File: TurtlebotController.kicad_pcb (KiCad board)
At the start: 2 copper layers, 110 x 80 mm, 80 parts, among them J1 Raspberry_Pi_2_3, J2 LEFT_MOTOR, J3 RIGHT_MOTOR, J4 5V_OUT, J5 3.3V _OUT, J6 12V_OUT, U1 Teensy4.0, U2 MinIMU-9_V5, U3 VNH5019, U4 VNH5019, U5 ACS711xLCTR-25AB, U6 D24V90F5, U7 UltimateSensorFusion_MPU9250_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

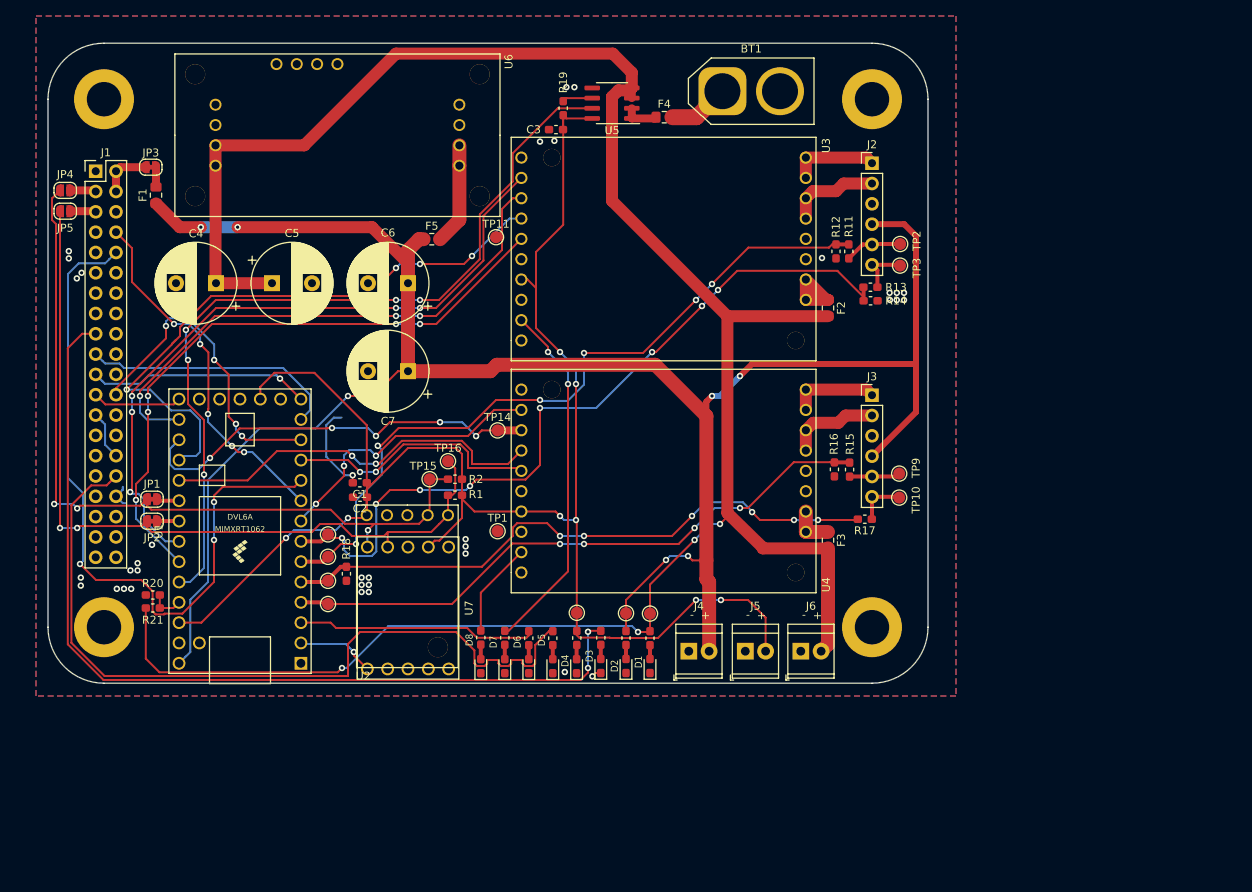
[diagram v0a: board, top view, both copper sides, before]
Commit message: Most of rev B
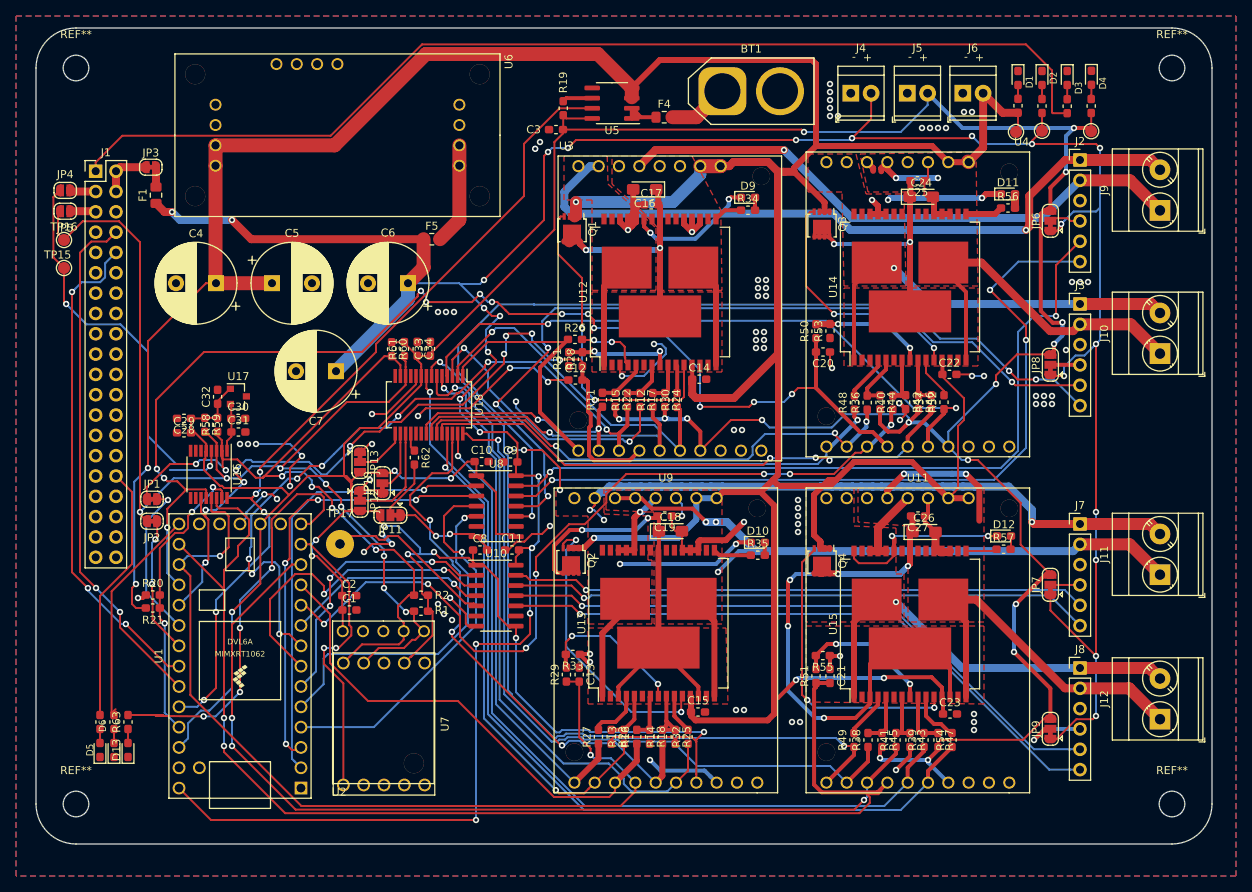
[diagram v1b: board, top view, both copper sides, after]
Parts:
- removed D7: LEFT_MOTOR_OK, LED_SMD:LED_0603_1608Metric_Pad1.05x0.95mm_HandSolder
- removed D8: RIGHT_MOTOR_OK, LED_SMD:LED_0603_1608Metric_Pad1.05x0.95mm_HandSolder
- removed F2, F3: Fuse, Fuse:Fuse_0805_2012Metric_Pad1.15x1.40mm_HandSolder
- removed R10, R9: 500Ohm, Resistor_SMD:R_0603_1608Metric_Pad1.05x0.95mm_HandSolder
- removed the REF** at (78.5, 111.4)
- removed the REF** at (174.5, 111.4)
- removed the REF** at (78.5, 45.4)
- removed the REF** at (174.5, 45.4)
- removed TP1: GND, TestPoint:TestPoint_Pad_D1.5mm
- removed TP10: RIGHT_ENCODER_B_5V, TestPoint:TestPoint_Pad_D1.5mm
- removed TP11: LEFT_PWM, TestPoint:TestPoint_Pad_D1.5mm
- removed TP12: RIGHT_ENCODER_A_3.3V, TestPoint:TestPoint_Pad_D1.5mm
- removed TP13: RIGHT_ENCODER_B_3.3V, TestPoint:TestPoint_Pad_D1.5mm
- removed TP14: RIGHT_PWM, TestPoint:TestPoint_Pad_D1.5mm
- removed TP2: LEFT_ENCODER_A_5V, TestPoint:TestPoint_Pad_D1.5mm
- removed TP3: LEFT_ENCODER_B_5V, TestPoint:TestPoint_Pad_D1.5mm
- removed TP7: LEFT_ENCODER_A_3.3V, TestPoint:TestPoint_Pad_D1.5mm
- removed TP8: LEFT_ENCODER_B_3.3V, TestPoint:TestPoint_Pad_D1.5mm
- removed TP9: RIGHT_ENCODER_A_5V, TestPoint:TestPoint_Pad_D1.5mm
- added C10: 0.1uF, Capacitor_SMD:C_0603_1608Metric_Pad1.05x0.95mm_HandSolder, F.Cu at (125.7, 90.7)
- added C11: 0.1uF, Capacitor_SMD:C_0603_1608Metric_Pad1.05x0.95mm_HandSolder, F.Cu at (129.5, 101.8)
- added C12: 33nF, Capacitor_SMD:C_0603_1608Metric_Pad1.05x0.95mm_HandSolder, F.Cu at (137.4, 80.5)
- added C13: 33nF, Capacitor_SMD:C_0603_1608Metric_Pad1.05x0.95mm_HandSolder, F.Cu at (137.9, 117.3)
- added C14: 0.1uF, Capacitor_SMD:C_0603_1608Metric_Pad1.05x0.95mm_HandSolder, F.Cu at (152.9, 80.4)
- added C15: 0.1uF, Capacitor_SMD:C_0603_1608Metric_Pad1.05x0.95mm_HandSolder, F.Cu at (152.8, 122.0)
- added C16: 47uF, Capacitor_Tantalum_SMD:CP_EIA-3216-10_Kemet-I_Pad1.58x1.35mm_HandSolder, F.Cu at (146.1, 56.7)
- added C17: 0.1uF, Capacitor_SMD:C_0603_1608Metric_Pad1.05x0.95mm_HandSolder, F.Cu at (146.9, 58.6)
- added C18: 47uF, Capacitor_Tantalum_SMD:CP_EIA-3216-10_Kemet-I_Pad1.58x1.35mm_HandSolder, F.Cu at (149.3, 99.4)
- added C19: 0.1uF, Capacitor_SMD:C_0603_1608Metric_Pad1.05x0.95mm_HandSolder, F.Cu at (148.6, 97.5)
- added C20: 33nF, Capacitor_SMD:C_0603_1608Metric_Pad1.05x0.95mm_HandSolder, F.Cu at (168.4, 77.0)
- added C21: 33nF, Capacitor_SMD:C_0603_1608Metric_Pad1.05x0.95mm_HandSolder, F.Cu at (169.2, 117.5)
- added C22: 0.1uF, Capacitor_SMD:C_0603_1608Metric_Pad1.05x0.95mm_HandSolder, F.Cu at (184.2, 79.8)
- added C23: 0.1uF, Capacitor_SMD:C_0603_1608Metric_Pad1.05x0.95mm_HandSolder, F.Cu at (184.2, 122.2)
- added C24: 47uF, Capacitor_Tantalum_SMD:CP_EIA-3216-10_Kemet-I_Pad1.58x1.35mm_HandSolder, F.Cu at (180.7, 57.6)
- added C25: 0.1uF, Capacitor_SMD:C_0603_1608Metric_Pad1.05x0.95mm_HandSolder, F.Cu at (180.2, 55.6)
- added C26: 47uF, Capacitor_Tantalum_SMD:CP_EIA-3216-10_Kemet-I_Pad1.58x1.35mm_HandSolder, F.Cu at (181.0, 99.5)
- added C27: 0.1uF, Capacitor_SMD:C_0603_1608Metric_Pad1.05x0.95mm_HandSolder, F.Cu at (180.2, 97.5)
- added C28: 1uF, Capacitor_SMD:C_0603_1608Metric_Pad1.05x0.95mm_HandSolder, F.Cu at (88.5, 85.3)
- added C29: 0.1uF, Capacitor_SMD:C_0603_1608Metric_Pad1.05x0.95mm_HandSolder, F.Cu at (88.5, 87.1)
- added C30: 0.1uF, Capacitor_SMD:C_0603_1608Metric_Pad1.05x0.95mm_HandSolder, F.Cu at (95.3, 85.3)
- added C31: 1uF, Capacitor_SMD:C_0603_1608Metric_Pad1.05x0.95mm_HandSolder, F.Cu at (95.3, 87.0)
- added C32: 0.47uF, Capacitor_SMD:C_0603_1608Metric_Pad1.05x0.95mm_HandSolder, F.Cu at (92.7, 82.6)
- added C33: 1uF, Capacitor_SMD:C_0603_1608Metric_Pad1.05x0.95mm_HandSolder, F.Cu at (119.3, 76.6)
- added C34: 0.1uF, Capacitor_SMD:C_0603_1608Metric_Pad1.05x0.95mm_HandSolder, F.Cu at (117.7, 76.6)
- added C8: 0.1uF, Capacitor_SMD:C_0603_1608Metric_Pad1.05x0.95mm_HandSolder, F.Cu at (125.5, 101.8)
- added C9: 0.1uF, Capacitor_SMD:C_0603_1608Metric_Pad1.05x0.95mm_HandSolder, F.Cu at (129.3, 90.8)
- added D10: LED_Dual_2pin, LED_SMD:LED_0603_1608Metric_Pad1.05x0.95mm_HandSolder, F.Cu at (160.2, 100.8)
- added D11: LED_Dual_2pin, LED_SMD:LED_0603_1608Metric_Pad1.05x0.95mm_HandSolder, F.Cu at (191.5, 57.2)
- added D12: LED_Dual_2pin, LED_SMD:LED_0603_1608Metric_Pad1.05x0.95mm_HandSolder, F.Cu at (191.0, 100.0)
- added D13: TEENSY_DEBUG, LED_SMD:LED_0603_1608Metric_Pad1.05x0.95mm_HandSolder, F.Cu at (81.5, 126.8)
- added D9: LED_Dual_2pin, LED_SMD:LED_0603_1608Metric_Pad1.05x0.95mm_HandSolder, F.Cu at (159.0, 57.7)
- added J10: Screw_Terminal_01x02, TerminalBlock_Phoenix:TerminalBlock_Phoenix_MKDS-3-2-5.08_1x02_P5.08mm_Horizontal, F.Cu at (210.5, 77.2)
- added J11: Screw_Terminal_01x02, TerminalBlock_Phoenix:TerminalBlock_Phoenix_MKDS-3-2-5.08_1x02_P5.08mm_Horizontal, F.Cu at (210.5, 104.8)
- added J12: Screw_Terminal_01x02, TerminalBlock_Phoenix:TerminalBlock_Phoenix_MKDS-3-2-5.08_1x02_P5.08mm_Horizontal, F.Cu at (210.5, 122.9)
- added J7: MOTOR_3, Connector_PinHeader_2.54mm:PinHeader_1x06_P2.54mm_Vertical, F.Cu at (200.5, 98.5)
- added J8: MOTOR_4, Connector_PinHeader_2.54mm:PinHeader_1x06_P2.54mm_Vertical, F.Cu at (200.5, 116.5)
- added J9: Screw_Terminal_01x02, TerminalBlock_Phoenix:TerminalBlock_Phoenix_MKDS-3-2-5.08_1x02_P5.08mm_Horizontal, F.Cu at (210.5, 59.3)
- added JP10: Jumper_3_Bridged12, Jumper:SolderJumper-3_P1.3mm_Bridged12_RoundedPad1.0x1.5mm, F.Cu at (113.3, 93.4)
- added JP11: Jumper_3_Bridged12, Jumper:SolderJumper-3_P1.3mm_Bridged12_RoundedPad1.0x1.5mm, F.Cu at (114.3, 97.4)
- added JP12: Jumper_3_Bridged12, Jumper:SolderJumper-3_P1.3mm_Bridged12_RoundedPad1.0x1.5mm, F.Cu at (110.5, 95.6)
- added JP13: Jumper_3_Bridged12, Jumper:SolderJumper-3_P1.3mm_Bridged12_RoundedPad1.0x1.5mm, F.Cu at (110.5, 90.8)
- added JP6: Jumper_3_Bridged12, Jumper:SolderJumper-3_P1.3mm_Bridged12_RoundedPad1.0x1.5mm, F.Cu at (196.8, 60.6)
- added JP7: Jumper_3_Bridged12, Jumper:SolderJumper-3_P1.3mm_Bridged12_RoundedPad1.0x1.5mm, F.Cu at (196.8, 106.1)
- added JP8: Jumper_3_Bridged12, Jumper:SolderJumper-3_P1.3mm_Bridged12_RoundedPad1.0x1.5mm, F.Cu at (196.8, 78.6)
- added JP9: Jumper_3_Bridged12, Jumper:SolderJumper-3_P1.3mm_Bridged12_RoundedPad1.0x1.5mm, F.Cu at (196.8, 124.1)
- added Q1: BUK7M12-40EX, Package_TO_SOT_SMD:LFPAK33, F.Cu at (137.0, 61.6)
- added Q2: BUK7M12-40EX, Package_TO_SOT_SMD:LFPAK33, F.Cu at (136.9, 103.0)
- added Q3: BUK7M12-40EX, Package_TO_SOT_SMD:LFPAK33, F.Cu at (168.2, 61.0)
- added Q4: BUK7M12-40EX, Package_TO_SOT_SMD:LFPAK33, F.Cu at (168.2, 103.1)
- added R22: 4.7k, Resistor_SMD:R_0603_1608Metric_Pad1.05x0.95mm_HandSolder, F.Cu at (142.4, 83.0)
- added R23: 4.7k, Resistor_SMD:R_0603_1608Metric_Pad1.05x0.95mm_HandSolder, F.Cu at (141.9, 125.1)
- added R24: 4.7k, Resistor_SMD:R_0603_1608Metric_Pad1.05x0.95mm_HandSolder, F.Cu at (148.6, 83.0)
- added R25: 4.7k, Resistor_SMD:R_0603_1608Metric_Pad1.05x0.95mm_HandSolder, F.Cu at (149.9, 125.1)
- added R26: 1k, Resistor_SMD:R_0603_1608Metric_Pad1.05x0.95mm_HandSolder, F.Cu at (137.4, 75.4)
- added R27: 1k, Resistor_SMD:R_0603_1608Metric_Pad1.05x0.95mm_HandSolder, F.Cu at (140.3, 125.1)
- added R28: 10k, Resistor_SMD:R_0603_1608Metric_Pad1.05x0.95mm_HandSolder, F.Cu at (138.3, 77.9)
- added R29: 10k, Resistor_SMD:R_0603_1608Metric_Pad1.05x0.95mm_HandSolder, F.Cu at (136.3, 117.3)
- added R30: 1k, Resistor_SMD:R_0603_1608Metric_Pad1.05x0.95mm_HandSolder, F.Cu at (150.2, 83.0)
- added R31: 1k, Resistor_SMD:R_0603_1608Metric_Pad1.05x0.95mm_HandSolder, F.Cu at (136.6, 77.9)
- added R32: 1k, Resistor_SMD:R_0603_1608Metric_Pad1.05x0.95mm_HandSolder, F.Cu at (151.5, 125.1)
- added R33: 1k, Resistor_SMD:R_0603_1608Metric_Pad1.05x0.95mm_HandSolder, F.Cu at (137.1, 114.8)
- added R34: 4.7k, Resistor_SMD:R_0603_1608Metric_Pad1.05x0.95mm_HandSolder, F.Cu at (159.0, 59.3)
- added R35: 4.7k, Resistor_SMD:R_0603_1608Metric_Pad1.05x0.95mm_HandSolder, F.Cu at (160.2, 102.4)
- added R36: 1k, Resistor_SMD:R_0603_1608Metric_Pad1.05x0.95mm_HandSolder, F.Cu at (173.9, 83.3)
- added R37: 1k, Resistor_SMD:R_0603_1608Metric_Pad1.05x0.95mm_HandSolder, F.Cu at (181.9, 83.3)
- added R38: 1k, Resistor_SMD:R_0603_1608Metric_Pad1.05x0.95mm_HandSolder, F.Cu at (174.0, 125.5)
- added R39: 1k, Resistor_SMD:R_0603_1608Metric_Pad1.05x0.95mm_HandSolder, F.Cu at (181.0, 125.5)
- added R40: 1k, Resistor_SMD:R_0603_1608Metric_Pad1.05x0.95mm_HandSolder, F.Cu at (177.1, 83.3)
- added R41: 1k, Resistor_SMD:R_0603_1608Metric_Pad1.05x0.95mm_HandSolder, F.Cu at (177.5, 125.5)
- added R42: 10k, Resistor_SMD:R_0603_1608Metric_Pad1.05x0.95mm_HandSolder, F.Cu at (178.7, 83.3)
- added R43: 10k, Resistor_SMD:R_0603_1608Metric_Pad1.05x0.95mm_HandSolder, F.Cu at (179.2, 125.5)
- added R44: 4.7k, Resistor_SMD:R_0603_1608Metric_Pad1.05x0.95mm_HandSolder, F.Cu at (175.5, 83.3)
- added R45: 4.7k, Resistor_SMD:R_0603_1608Metric_Pad1.05x0.95mm_HandSolder, F.Cu at (175.8, 125.5)
- added R46: 4.7k, Resistor_SMD:R_0603_1608Metric_Pad1.05x0.95mm_HandSolder, F.Cu at (180.3, 83.3)
- added R47: 4.7k, Resistor_SMD:R_0603_1608Metric_Pad1.05x0.95mm_HandSolder, F.Cu at (182.8, 125.5)
- added R48: 1k, Resistor_SMD:R_0603_1608Metric_Pad1.05x0.95mm_HandSolder, F.Cu at (172.3, 83.3)
- added R49: 1k, Resistor_SMD:R_0603_1608Metric_Pad1.05x0.95mm_HandSolder, F.Cu at (172.2, 125.5)
- added R50: 10k, Resistor_SMD:R_0603_1608Metric_Pad1.05x0.95mm_HandSolder, F.Cu at (167.5, 74.4)
- added R51: 10k, Resistor_SMD:R_0603_1608Metric_Pad1.05x0.95mm_HandSolder, F.Cu at (167.5, 117.5)
- added R52: 1k, Resistor_SMD:R_0603_1608Metric_Pad1.05x0.95mm_HandSolder, F.Cu at (183.5, 83.3)
- added R53: 1k, Resistor_SMD:R_0603_1608Metric_Pad1.05x0.95mm_HandSolder, F.Cu at (169.2, 74.4)
- added R54: 1k, Resistor_SMD:R_0603_1608Metric_Pad1.05x0.95mm_HandSolder, F.Cu at (184.5, 125.5)
- added R55: 1k, Resistor_SMD:R_0603_1608Metric_Pad1.05x0.95mm_HandSolder, F.Cu at (168.3, 115.0)
- added R56: 4.7k, Resistor_SMD:R_0603_1608Metric_Pad1.05x0.95mm_HandSolder, F.Cu at (191.5, 59.0)
- added R57: 4.7k, Resistor_SMD:R_0603_1608Metric_Pad1.05x0.95mm_HandSolder, F.Cu at (190.9, 101.7)
- added R58: 4.7k, Resistor_SMD:R_0603_1608Metric_Pad1.05x0.95mm_HandSolder, F.Cu at (92.7, 86.1)
- added R59: 4.7k, Resistor_SMD:R_0603_1608Metric_Pad1.05x0.95mm_HandSolder, F.Cu at (91.1, 86.1)
- added R60: 4.7k, Resistor_SMD:R_0603_1608Metric_Pad1.05x0.95mm_HandSolder, F.Cu at (114.5, 76.7)
- added R61: 4.7k, Resistor_SMD:R_0603_1608Metric_Pad1.05x0.95mm_HandSolder, F.Cu at (116.0, 76.6)
- added R62: 4.7k, Resistor_SMD:R_0603_1608Metric_Pad1.05x0.95mm_HandSolder, F.Cu at (117.3, 90.2)
- added R63: 65Ohm, Resistor_SMD:R_0603_1608Metric_Pad1.05x0.95mm_HandSolder, F.Cu at (81.5, 123.2)
- added REF**: MountingHole_3.2mm_M3, MountingHole:MountingHole_3.2mm_M3, F.Cu at (212.0, 133.5)
- added REF**: MountingHole_3.2mm_M3, MountingHole:MountingHole_3.2mm_M3, F.Cu at (75.0, 133.5)
- added REF**: MountingHole_3.2mm_M3, MountingHole:MountingHole_3.2mm_M3, F.Cu at (212.0, 41.5)
- added REF**: MountingHole_3.2mm_M3, MountingHole:MountingHole_3.2mm_M3, F.Cu at (75.0, 41.5)
- added TP17: TestPoint, Connector_Wire:SolderWirePad_1x01_Drill1.2mm, F.Cu at (108.0, 101.0)
- added U10: TXB0104D, Package_SO:SOIC-14_3.9x8.7mm_P1.27mm, F.Cu at (127.5, 107.5)
- added U11: VNH5019, TurtlebotController:Pololu_VNH5019_Carrier, F.Cu at (181.5, 94.0)
- added U12: VNH5019A-E, Package_SO:ST_MultiPowerSO-30, F.Cu at (148.0, 69.5)
- added U13: VNH5019A-E, Package_SO:ST_MultiPowerSO-30, F.Cu at (147.8, 110.9)
- added U14: VNH5019A-E, Package_SO:ST_MultiPowerSO-30, F.Cu at (179.2, 68.9)
- added U15: VNH5019A-E, Package_SO:ST_MultiPowerSO-30, F.Cu at (179.2, 111.0)
- added U16: ADC128D818, Package_SO:TSSOP-16_4.4x5mm_P0.65mm, F.Cu at (91.6, 92.3)
- added U17: REF3030, Package_TO_SOT_SMD:SOT-23, F.Cu at (95.3, 82.5)
- added U18: MCP23017_SS, Package_SO:SSOP-28_5.3x10.2mm_P0.65mm, F.Cu at (119.1, 83.6)
- added U8: TXB0104D, Package_SO:SOIC-14_3.9x8.7mm_P1.27mm, F.Cu at (127.5, 96.3)
- added U9: VNH5019, TurtlebotController:Pololu_VNH5019_Carrier, F.Cu at (150.0, 94.0)
- J2: value LEFT_MOTOR -> MOTOR_1
- J3: value RIGHT_MOTOR -> MOTOR_2
- R11, R13, R15: value 270Ohm -> 1k
- R12, R14, R16: value 560Ohm -> 1k
- R17: value 270Ohm -> 10k
- R18: value 560Ohm -> 10k
- moved D4 97.7 mm to (201.9, 42.7), turned to 270 degrees
- moved D3 93.8 mm to (198.9, 42.8), turned to 270 degrees
- moved R6 92.5 mm to (201.9, 46.2), turned to 270 degrees
- moved D2 90.0 mm to (195.8, 42.8), turned to 270 degrees
- moved R5 88.4 mm to (198.9, 46.3), turned to 270 degrees
- moved TP4 88.1 mm to (201.9, 49.4), turned to 180 degrees
- moved D1 86.7 mm to (192.8, 42.8), turned to 270 degrees
- moved R4 84.4 mm to (195.8, 46.2), turned to 270 degrees
- moved R3 80.9 mm to (192.8, 46.2), turned to 270 degrees
- moved TP5 79.6 mm to (195.8, 49.4), turned to 180 degrees
- moved TP6 75.6 mm to (192.5, 49.5), turned to 180 degrees
- moved J4 72.6 mm to (171.8, 44.6)
- moved J5 72.6 mm to (178.9, 44.6)
- moved J6 72.6 mm to (185.8, 44.6)
- moved R13 64.1 mm to (143.5, 125.1), turned to 90 degrees
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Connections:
- net LEFT_MOTOR_A renamed MOTOR_1_A
- net LEFT_MOTOR_B renamed MOTOR_1_B
- net RIGHT_MOTOR_A renamed MOTOR_2_A
- net RIGHT_MOTOR_B renamed MOTOR_2_B
- J1 pad 11: Net-(J1-Pad11) -> (no net)
- J1 pad 12: Net-(J1-Pad12) -> (no net)
- J1 pad 13: Net-(J1-Pad13) -> (no net)
- J1 pad 15: Net-(J1-Pad15) -> (no net)
- J1 pad 16: Net-(J1-Pad16) -> (no net)
- J1 pad 18: Net-(J1-Pad18) -> (no net)
- J1 pad 19: TEENSY_MOSI -> (no net)
- J1 pad 21: TEENSY_MISO -> (no net)
- J1 pad 22: Net-(J1-Pad22) -> (no net)
- J1 pad 23: TEENSY_SCK -> (no net)
- J1 pad 24: TEENSY_CS -> (no net)
- J1 pad 26: Net-(J1-Pad26) -> (no net)
- J1 pad 27: Net-(J1-Pad27) -> (no net)
- J1 pad 28: Net-(J1-Pad28) -> (no net)
- J1 pad 29: Net-(J1-Pad29) -> (no net)
- J1 pad 31: Net-(J1-Pad31) -> (no net)
- J1 pad 33: Net-(J1-Pad33) -> (no net)
- J1 pad 35: Net-(J1-Pad35) -> (no net)
- J1 pad 36: Net-(J1-Pad36) -> (no net)
- J1 pad 37: Net-(J1-Pad37) -> (no net)
- J1 pad 38: Net-(J1-Pad38) -> (no net)
- J1 pad 40: Net-(J1-Pad40) -> (no net)
- J1 pad 7: Net-(J1-Pad7) -> (no net)
- J2 pad 4: +5V -> Net-(J2-Pad4)
- J2 pad 5: LEFT_ENCODER_A_5V -> MOTOR_1_ENCODER_A_5V
- J2 pad 6: LEFT_ENCODER_B_5V -> MOTOR_1_ENCODER_B_5V
- J3 pad 4: +5V -> Net-(J3-Pad4)
- J3 pad 5: RIGHT_ENCODER_A_5V -> MOTOR_2_ENCODER_A_5V
- J3 pad 6: RIGHT_ENCODER_B_5V -> MOTOR_2_ENCODER_B_5V
- R11 pad 1: LEFT_ENCODER_A_5V -> MOTOR_1_DIAGA
- R11 pad 2: LEFT_ENCODER_A_3.3V -> Net-(R11-Pad2)
- R12 pad 1: LEFT_ENCODER_A_3.3V -> MOTOR_1_DIAGB
- R12 pad 2: GND -> Net-(R12-Pad2)
- R13 pad 1: LEFT_ENCODER_B_5V -> MOTOR_3_DIAGA
- R13 pad 2: LEFT_ENCODER_B_3.3V -> Net-(R13-Pad2)
- R14 pad 1: LEFT_ENCODER_B_3.3V -> MOTOR_3_DIAGB
- R14 pad 2: GND -> Net-(R14-Pad2)
- R15 pad 1: RIGHT_ENCODER_A_5V -> MOTOR_1_PWM
- R15 pad 2: RIGHT_ENCODER_A_3.3V -> Net-(R15-Pad2)
- R16 pad 1: RIGHT_ENCODER_A_3.3V -> MOTOR_3_PWM
- R16 pad 2: GND -> Net-(R16-Pad2)
- R17 pad 1: RIGHT_ENCODER_B_5V -> Net-(R15-Pad2)
- R17 pad 2: RIGHT_ENCODER_B_3.3V -> GND
- R18 pad 1: RIGHT_ENCODER_B_3.3V -> Net-(R16-Pad2)
- U1 pad 10: TEENSY_TX -> MOTOR_2_PWM
- U1 pad 11: RIGHT_MOTOR_DIAGB -> MOTOR_3_PWM
- U1 pad 12: TEENSY_CS -> MOTOR_4_PWM
- U1 pad 13: TEENSY_MOSI -> MPU_INTERRUPT
- U1 pad 14: TEENSY_MISO -> TEENSY_DEBUG
- U1 pad 15: Net-(U1-Pad15) -> (no net)
- U1 pad 18: Net-(U1-Pad18) -> (no net)
- U1 pad 19: Net-(U1-Pad19) -> (no net)
- U1 pad 2: MPU_INTERRUPT -> MOTOR_1_ENCODER_A
- U1 pad 20: TEENSY_SCK -> TEENSY_HEARTBEAT
- U1 pad 21: LEFT_MOTOR_PWM -> MOTOR_4_CS
- U1 pad 22: RIGHT_MOTOR_PWM -> MOTOR_3_CS
- U1 pad 23: LEFT_MOTOR_CURRENT -> MOTOR_2_CS
- U1 pad 24: RIGHT_MOTOR_CURRENT -> MOTOR_1_CS
- U1 pad 27: LEFT_MOTOR_DIAGA -> TEENSY_TX
- U1 pad 28: LEFT_MOTOR_DIAGB -> TEENSY_RX
- U1 pad 3: TEENSY_HEARTBEAT -> MOTOR_1_ENCODER_B
- U1 pad 34: Net-(U1-Pad34) -> (no net)
- U1 pad 4: RIGHT_ENCODER_A_3.3V -> MOTOR_2_ENCODER_A
- U1 pad 5: RIGHT_ENCODER_B_3.3V -> MOTOR_2_ENCODER_B
- U1 pad 6: LEFT_ENCODER_A_3.3V -> MOTOR_3_ENCODER_A
- U1 pad 7: LEFT_ENCODER_B_3.3V -> MOTOR_3_ENCODER_B
- U1 pad 8: RIGHT_MOTOR_DIAGA -> MOTOR_1_PWM
- U1 pad 9: TEENSY_RX -> MOTOR_4_ENCODER_A
- U2 pad 4: Net-(U2-Pad4) -> (no net)
- U3 pad 1: Net-(U3-Pad1) -> MOTOR_1_INA
- U3 pad 14: Net-(F2-Pad1) -> +12V
- U3 pad 2: LEFT_MOTOR_DIAGA -> MOTOR_1_DIAGA
- U3 pad 3: LEFT_MOTOR_PWM -> MOTOR_1_PWM
- U3 pad 4: LEFT_MOTOR_CURRENT -> MOTOR_1_CS
- U3 pad 5: LEFT_MOTOR_DIAGB -> MOTOR_1_DIAGB
- U3 pad 6: Net-(U3-Pad6) -> MOTOR_1_INB
- U3 pad 9: LEFT_MOTOR_OUT -> (no net)
- U4 pad 1: Net-(U4-Pad1) -> MOTOR_2_INA
- U4 pad 14: Net-(F3-Pad1) -> +12V
- U4 pad 2: RIGHT_MOTOR_DIAGA -> MOTOR_2_DIAGA
- U4 pad 3: RIGHT_MOTOR_PWM -> MOTOR_2_PWM
- U4 pad 4: RIGHT_MOTOR_CURRENT -> MOTOR_2_CS
- U4 pad 5: RIGHT_MOTOR_DIAGB -> MOTOR_2_DIAGB
- U4 pad 6: Net-(U4-Pad6) -> MOTOR_2_INB
- U4 pad 9: RIGHT_MOTOR_OUT -> (no net)
- U6 pad 5: Net-(U6-Pad5) -> (no net)
- U6 pad 6: 5v_PG -> (no net)
- U6 pad 7: Net-(U6-Pad7) -> (no net)
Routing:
- net +3V3: track 212.4 -> 562.8 mm, vias 8 -> 26
- net GND: track 22.2 -> 232.8 mm, vias 36 -> 99
- net +12V: track 278.6 -> 465.6 mm, vias 4 -> 6
- net MOTOR_4_CS: track 0.00 -> 157.8 mm, vias 0 -> 2
- net MOTOR_2_CS: track 0.00 -> 148.6 mm, vias 0 -> 13
- net +5V: track 262.1 -> 400.2 mm, vias 7 -> 27
- net MOTOR_4_PWM: track 0.00 -> 118.0 mm, vias 0 -> 3
- net MOTOR_3_CS: track 0.00 -> 113.5 mm, vias 0 -> 2
- net MOTOR_4_INB: track 0.00 -> 112.5 mm, vias 0 -> 1
- net MOTOR_2_ENCODER_B_5V: track 0.00 -> 112.3 mm, vias 0 -> 3
- net MOTOR_3_A: track 0.00 -> 109.6 mm, vias 0 -> 6
- net MOTOR_1_A: track 11.1 -> 119.4 mm, vias 0 -> 3
- net MOTOR_2_ENCODER_A_5V: track 0.00 -> 104.0 mm, vias 0 -> 4
- net MOTOR_2_PWM: track 0.00 -> 102.2 mm, vias 0 -> 7
- net LEFT_ENCODER_B_3.3V: track 101.4 -> 0.00 mm, vias 8 -> 0
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- added copper zone on F.Cu, net MOTOR_1_A
- added copper zone on F.Cu, net MOTOR_1_B
- added copper zone on F.Cu, net MOTOR_2_A
- added copper zone on F.Cu, net MOTOR_2_B
- added copper zone on F.Cu, net MOTOR_3_A
- added copper zone on F.Cu, net MOTOR_3_B
- added copper zone on F.Cu, net MOTOR_4_A
- added copper zone on F.Cu, net MOTOR_4_B
- added copper zone on F.Cu, net Net-(C16-Pad1)
- added copper zone on F.Cu, net Net-(C18-Pad1)
- added copper zone on F.Cu, net Net-(C24-Pad1)
- added copper zone on F.Cu, net Net-(C26-Pad1)
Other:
- board size 110 x 80 mm -> 147 x 102 mm
